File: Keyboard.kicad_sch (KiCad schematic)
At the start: 39 parts, among them J1 USB_C_Receptacle, J2 Conn_02x01, J4 FFC2B35-16-G_REVA2, Q1 PMOS, Q2 NMOS, Q3 NMOS, U1 VBUS54CV-HSF-G4-08, U3 MCP73831-2-OT, U4 LM1117DT-3.3, U5 ESP32-S3-WROOM-1-N16R2

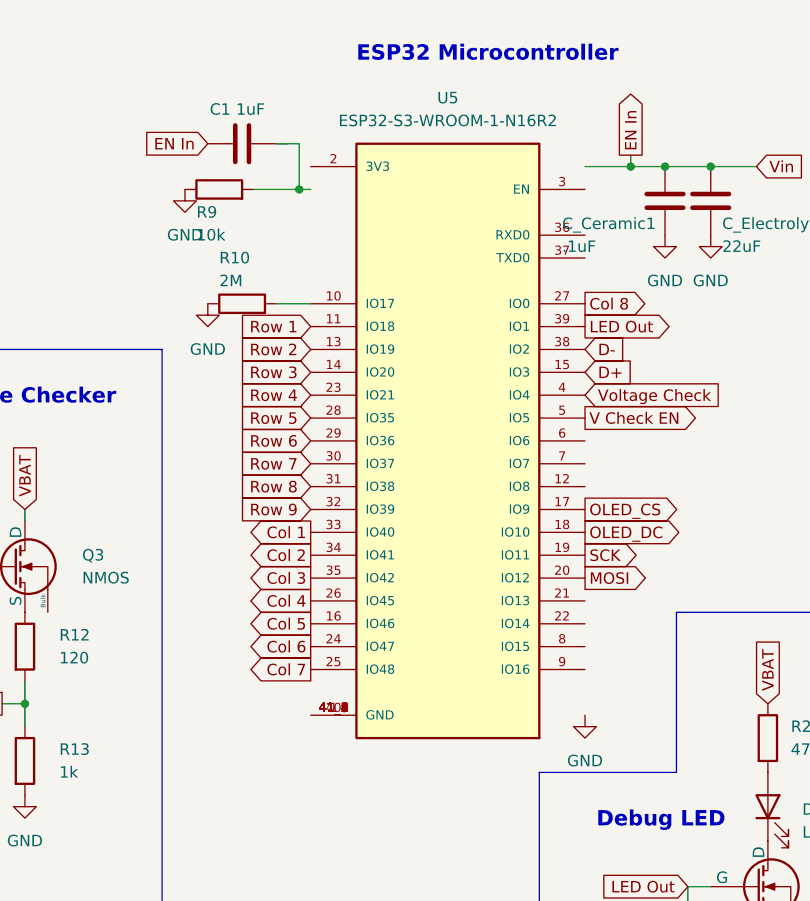
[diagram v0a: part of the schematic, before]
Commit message: made further progress on the keyboard pcb
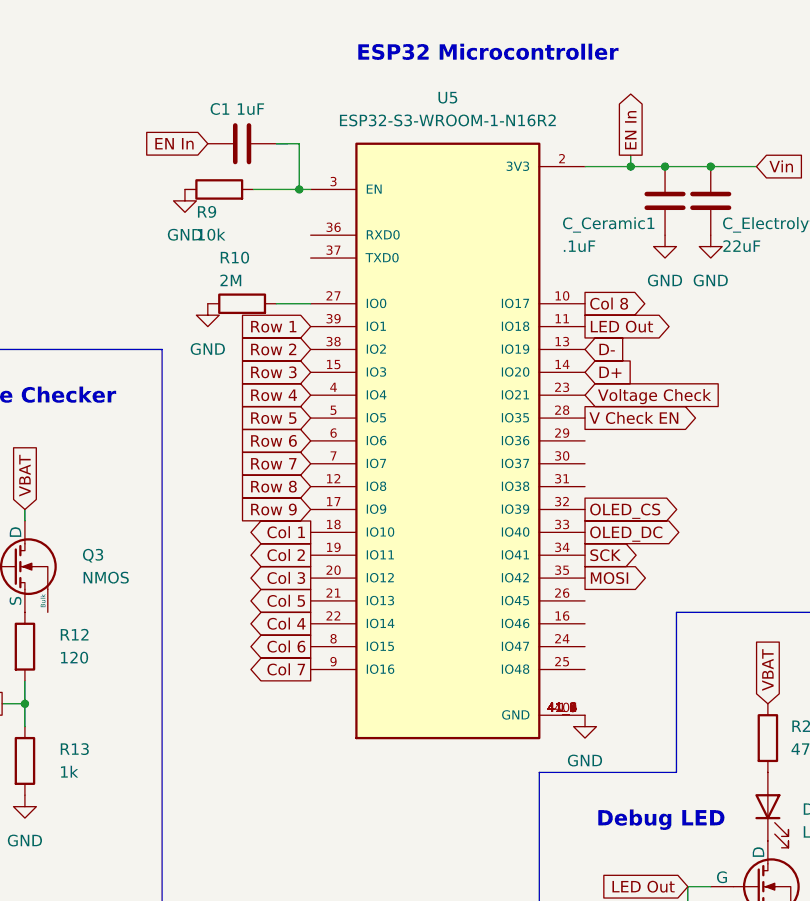
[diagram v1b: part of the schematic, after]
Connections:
- net Col 1: now also U5.18 (IO10); no longer U5.33 (IO40)
- net Col 2: now also U5.19 (IO11); no longer U5.34 (IO41)
- net Col 3: now also U5.20 (IO12); no longer U5.35 (IO42)
- net Col 4: now also U5.22 (IO14); no longer U5.26 (IO45)
- net Col 5: now also U5.21 (IO13); no longer U5.16 (IO46)
- net Col 6: now also U5.8 (IO15); no longer U5.24 (IO47)
- net Col 7: now also U5.9 (IO16); no longer U5.25 (IO48)
- net Col 8: now also U5.10 (IO17); no longer U5.27 (IO0)
- net D+: now also U5.14 (IO20); no longer U5.15 (IO3)
- net D-: now also U5.13 (IO19); no longer U5.38 (IO2)
- net EN In: now also U5.2 (3V3)
- net GND: now also U5.1 (GND), U5.40 (GND), U5.41_1 (GND), U5.41_2 (GND), U5.41_3 (GND), U5.41_4 (GND), U5.41_5 (GND), U5.41_6 (GND), U5.41_7 (GND), U5.41_8 (GND), U5.41_9 (GND)
- net LED Out: now also U5.11 (IO18); no longer U5.39 (IO1)
- net MOSI: now also U5.35 (IO42); no longer U5.20 (IO12)
- net OLED_CS: now also U5.32 (IO39); no longer U5.17 (IO9)
- net OLED_DC: now also U5.33 (IO40); no longer U5.18 (IO10)
- net Row 1: now also U5.39 (IO1); no longer U5.11 (IO18)
- net Row 2: now also U5.38 (IO2); no longer U5.13 (IO19)
- net Row 3: now also U5.15 (IO3); no longer U5.14 (IO20)
- net Row 4: now also U5.4 (IO4); no longer U5.23 (IO21)
- net Row 5: now also U5.5 (IO5); no longer U5.28 (IO35)
- net Row 6: now also U5.6 (IO6); no longer U5.29 (IO36)
- net Row 7: now also U5.7 (IO7); no longer U5.30 (IO37)
- net Row 8: now also U5.12 (IO8); no longer U5.31 (IO38)
- net Row 9: now also U5.17 (IO9); no longer U5.32 (IO39)
- net SCK: now also U5.34 (IO41); no longer U5.19 (IO11)
- net V Check EN: now also U5.28 (IO35); no longer U5.5 (IO5)
- net Voltage Check: now also U5.23 (IO21); no longer U5.4 (IO4)
- net at R10.2: now also U5.27 (IO0); no longer U5.10 (IO17)
- net at U5.3 (EN): now also C1.2, R9.2
